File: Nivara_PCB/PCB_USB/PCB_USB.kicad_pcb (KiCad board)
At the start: 2 copper layers, 33.4 x 18 mm, 6 parts, among them J1 PINHD_2x2_Male, U1 GT-USB-7010ASV

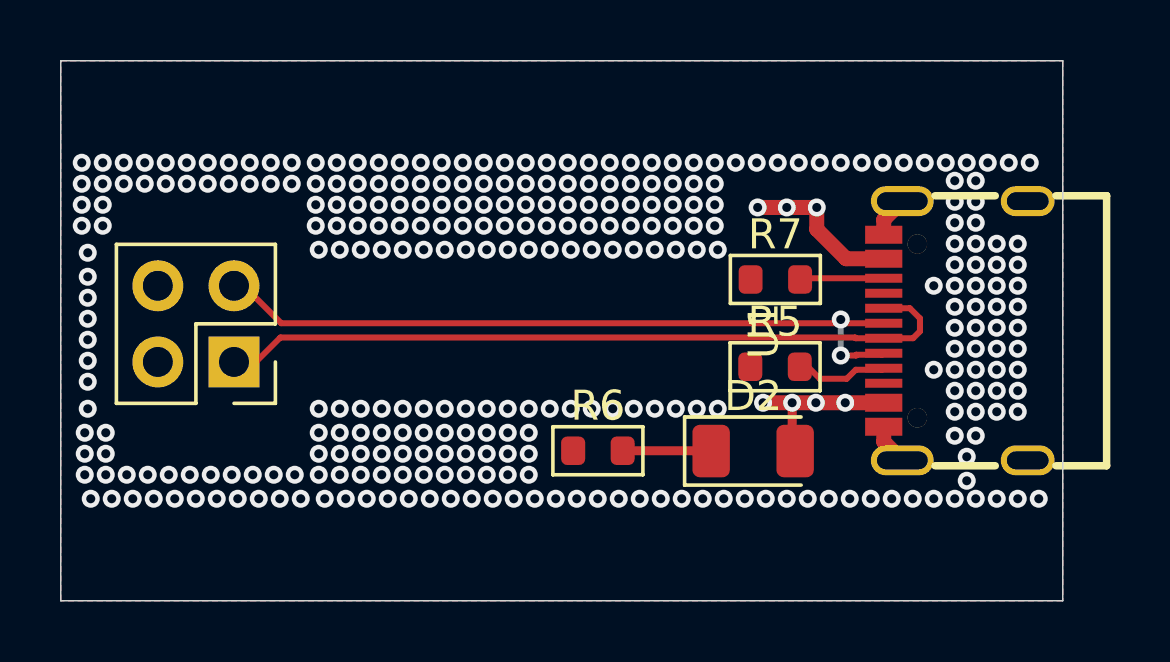
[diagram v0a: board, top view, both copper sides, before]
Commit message: S.
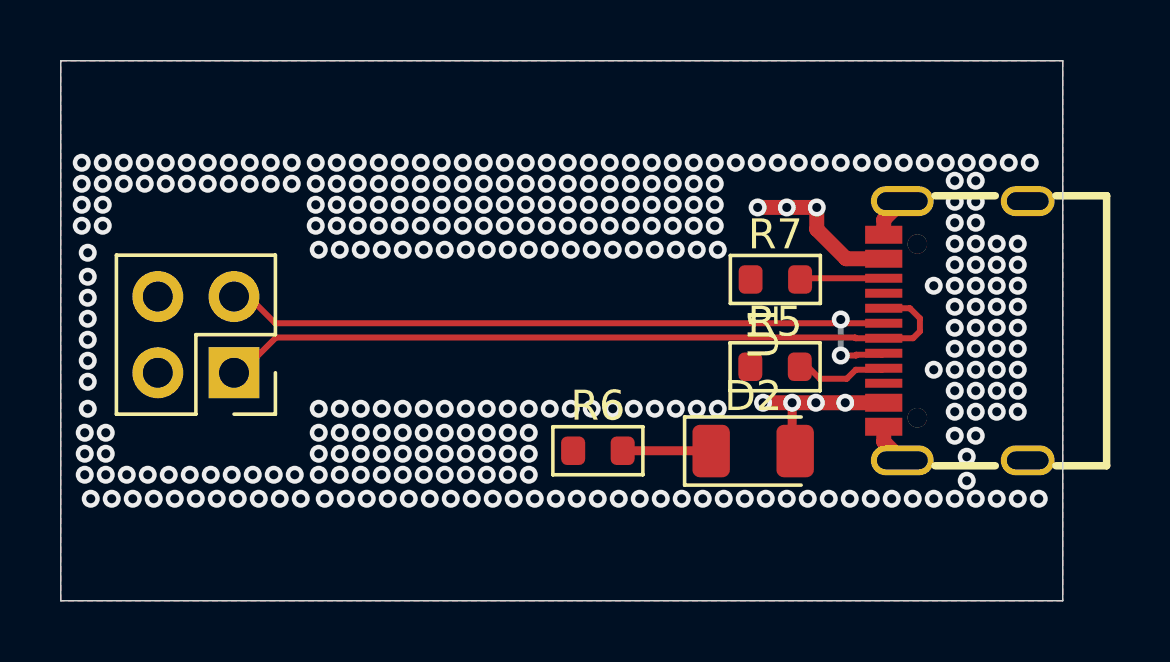
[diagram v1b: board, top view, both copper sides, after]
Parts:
- moved J1 0.36 mm to (107.4, 96.9)
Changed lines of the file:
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@@
 	(footprint "Connector_PinHeader_2.54mm:PinHeader_2x02_P2.54mm_Vertical"
 		(layer "F.Cu")
-		(at 107.375 96.54 180)
+		(at 107.375 96.9 180)
 		(descr "Through hole straight pin header, 2x02, 2.54mm pitch, double rows")
 		(tags "Through hole pin header THT 2x02 2.54mm double row")
@@
 	)
 	(segment
-		(start 107.835 94.135)
+		(start 129.0325 95.25)
+		(end 108.75 95.25)
+		(width 0.2)
+		(layer "F.Cu")
+		(net 7)
+	)
+	(segment
+		(start 108.75 95.25)
+		(end 107.86 94.36)
+		(width 0.2)
+		(layer "F.Cu")
+		(net 7)
+	)
+	(segment
+		(start 107.375 94.36)
 		(end 107.375 94.135)
 		(width 0.2)
@@
 	)
 	(segment
-		(start 108.95 95.25)
-		(end 107.835 94.135)
+		(start 107.86 94.36)
+		(end 107.375 94.36)
 		(width 0.2)
 		(layer "F.Cu")
@@
 		(net 7)
 	)
-	(segment
-		(start 129.0325 95.25)
-		(end 108.95 95.25)
-		(width 0.2)
-		(layer "F.Cu")
-		(net 7)
-	)
 	(via
 		(at 127.6 96.325)
@@
 	)
 	(segment
-		(start 129.0325 95.75)
-		(end 128.102499 95.75)
+		(start 128.102499 95.75)
+		(end 128.077499 95.725)
 		(width 0.2)
 		(layer "F.Cu")
@@
 	)
 	(segment
-		(start 128.102499 95.75)
-		(end 128.077499 95.725)
+		(start 107.825 96.675)
+		(end 107.775 96.675)
 		(width 0.2)
 		(layer "F.Cu")
@@
 	)
 	(segment
-		(start 107.970698 96.675)
-		(end 107.775 96.675)
+		(start 128.077499 95.725)
+		(end 108.775 95.725)
 		(width 0.2)
 		(layer "F.Cu")
@@
 	)
 	(segment
-		(start 108.920698 95.725)
-		(end 107.970698 96.675)
+		(start 129.0325 95.75)
+		(end 128.102499 95.75)
 		(width 0.2)
 		(layer "F.Cu")
@@
 	)
 	(segment
-		(start 130.01 95.75)
-		(end 129.0325 95.75)
+		(start 108.775 95.725)
+		(end 107.825 96.675)
 		(width 0.2)
 		(layer "F.Cu")
@@
 	)
 	(segment
-		(start 128.077499 95.725)
-		(end 108.920698 95.725)
+		(start 130.01 95.75)
+		(end 129.0325 95.75)
 		(width 0.2)
 		(layer "F.Cu")
